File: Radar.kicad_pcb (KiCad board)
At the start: 2 copper layers, 119 parts, among them J1 Receive_Antenna, J10 Conn_Coaxial, J11 Conn_02x05_Counter_Clockwise, J2 VCO_Tune, J3 Transmit Antenna, J4 Output, J5 Conn_Coaxial, J6 Conn_Coaxial, J7 Conn_Coaxial, J8 Conn_Coaxial, J9 Conn_Coaxial, U10 AD5252, U11 LT1722, U12 AD8039, U13 PMA-63GLN+, U14 QPC6324, U15 PMA-63GLN+, U16 QPC6324, U17 HMC218BMS8GE, U18 AZ1117-5.0, U19 RP117, U20 MIC5317, U21 L78L33_SO8, U23 HMC430, U24 RFPA5542

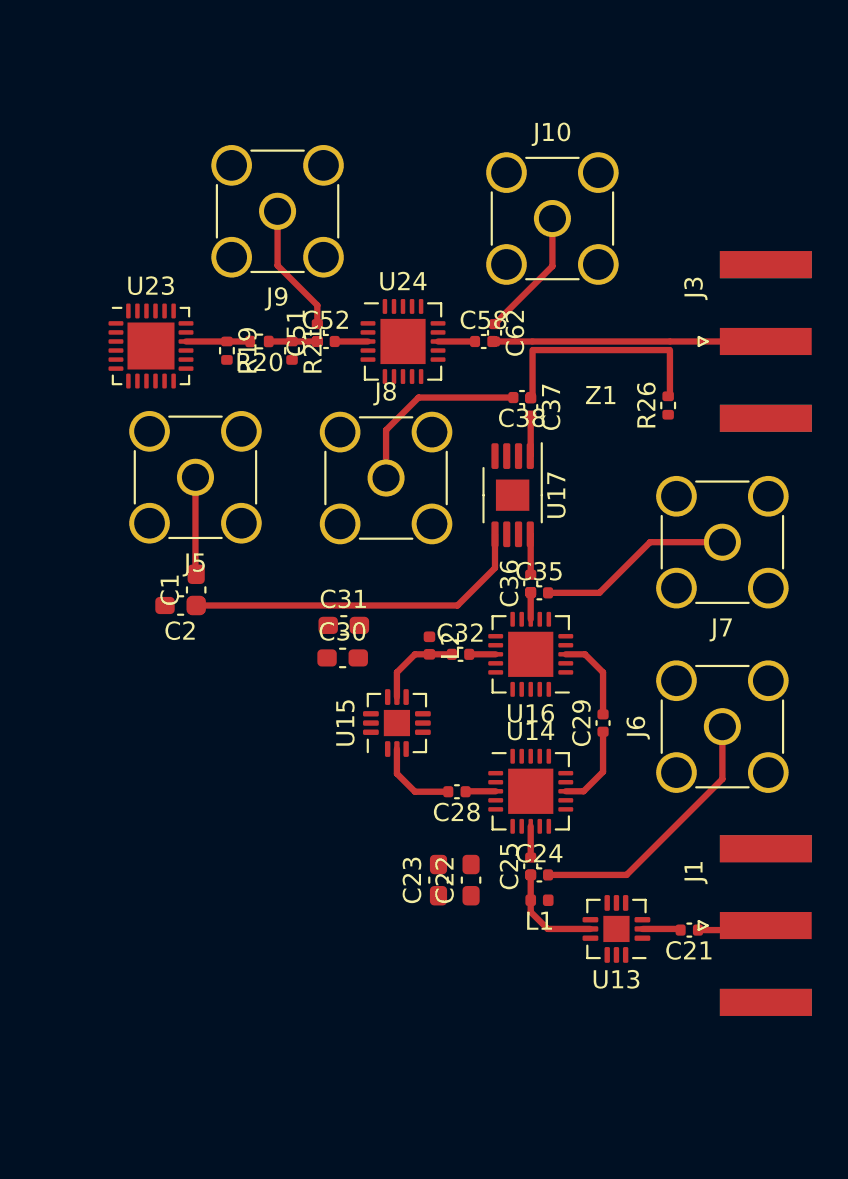
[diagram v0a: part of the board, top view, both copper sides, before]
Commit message: Curved tracks
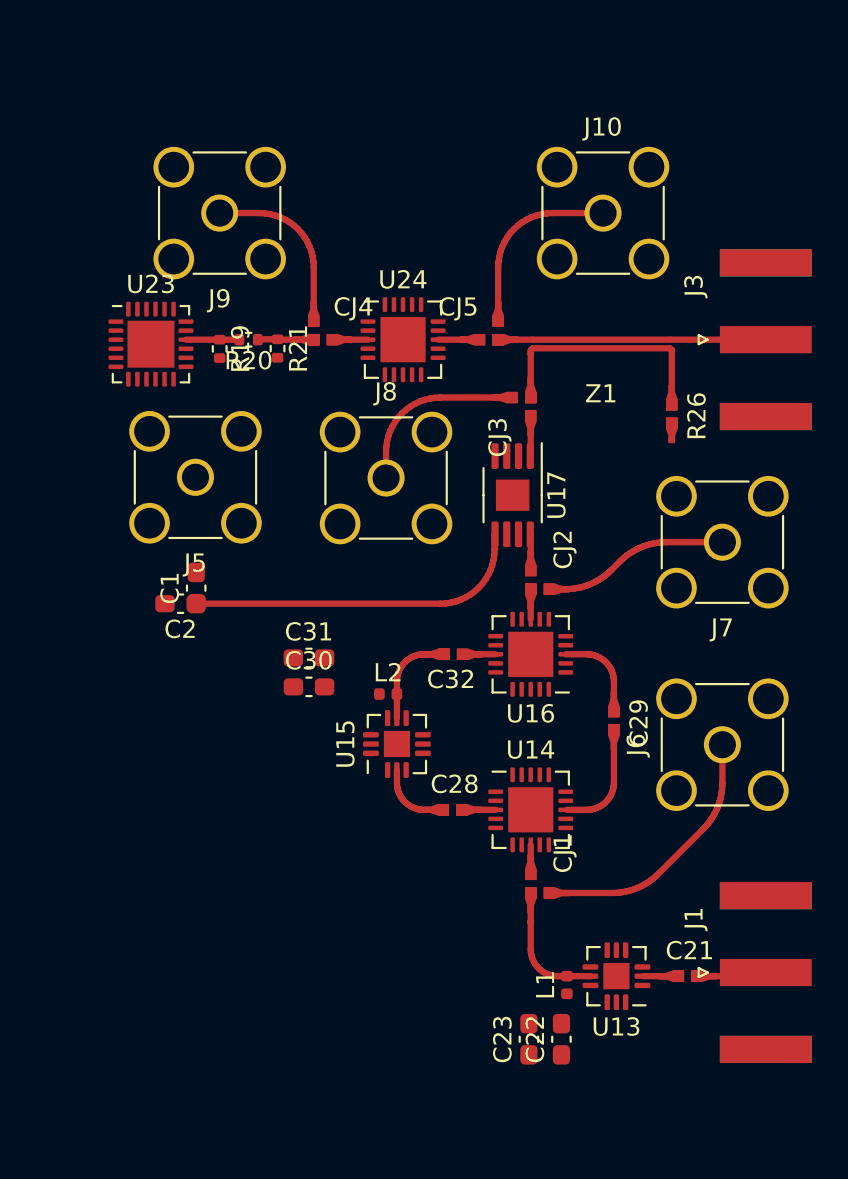
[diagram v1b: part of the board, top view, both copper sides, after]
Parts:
- removed C24, C35, C38, C51: DNP, Capacitor_SMD:C_0402_1005Metric
- removed C25, C36, C37, C52, C58, C62: 100pF, Capacitor_SMD:C_0402_1005Metric
- added CJ1: 100pF, own:0402_Jumper_Tapered, F.Cu at (162.0, 70.2)
- added CJ2: 100pF, own:0402_Jumper_Tapered, F.Cu at (162.0, 53.4)
- added CJ3: 100pF, own:0402_Jumper_Tapered, F.Cu at (162.0, 42.8)
- added CJ4: 100pF, own:0402_Jumper_Tapered, F.Cu at (150.8, 39.6)
- added CJ5: 100pF, own:0402_Jumper_Tapered, F.Cu at (160.2, 39.6)
- C21, C28, C29, C32: footprint Capacitor_SMD:C_0402_1005Metric -> own:0402_Tapered
- R26: footprint Resistor_SMD:R_0402_1005Metric -> own:0402_Tapered
- moved C22 10.1 mm to (163.7, 78.3)
- moved C23 10.1 mm to (161.9, 78.3)
- moved L1 4.92 mm to (164.0, 75.3), turned to 90 degrees
- moved L2 3.53 mm to (154.1, 59.2), turned to 0 degrees
- moved J9 3.20 mm to (144.8, 32.6)
- moved J10 2.82 mm to (166.0, 32.6)
- moved C31 2.64 mm to (149.7, 57.2)
- moved U13 2.61 mm to (166.7, 74.8)
- moved J1 2.60 mm to (175.0, 74.6)
- moved C21 2.59 mm to (171.2, 74.8), turned to 0 degrees
- moved C30 2.46 mm to (149.7, 58.8)
- moved U15 1.16 mm to (154.6, 62.0)
- moved C28 1.04 mm to (158.2, 65.6), turned to 0 degrees
- moved U14 1.02 mm to (162.0, 65.6)
- moved R26 1.01 mm to (169.8, 44.2), turned to 270 degrees
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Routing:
- net Net-(C1-Pad2): track 5.38 -> 0.00 mm
- net Net-(CJ5-Pad3): track 7.17 -> 10.5 mm
- net Net-(CJ4-Pad3): track 7.15 -> 9.88 mm
- net Net-(C28-Pad2): track 4.62 -> 3.06 mm
- net Net-(CJ1-Pad1): track 5.74 -> 7.27 mm
- net Net-(C32-Pad1): track 4.82 -> 5.63 mm
- net /Transmitter/RF_OUT: track 6.10 -> 5.30 mm
- net Net-(R19-Pad1): track 3.55 -> 2.95 mm
- net Net-(C29-Pad1): track 4.73 -> 5.33 mm
- net Net-(R26-Pad2): track 2.60 -> 3.17 mm
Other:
- net class Default: clearance 0.1 -> 0.09
- net class RF: clearance 0.1 -> 0.09
- rule trace_clearance: 0.1 -> 0.09
